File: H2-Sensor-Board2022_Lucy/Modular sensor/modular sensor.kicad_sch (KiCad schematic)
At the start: 6 parts, among them J1 Conn_01x03_Pin

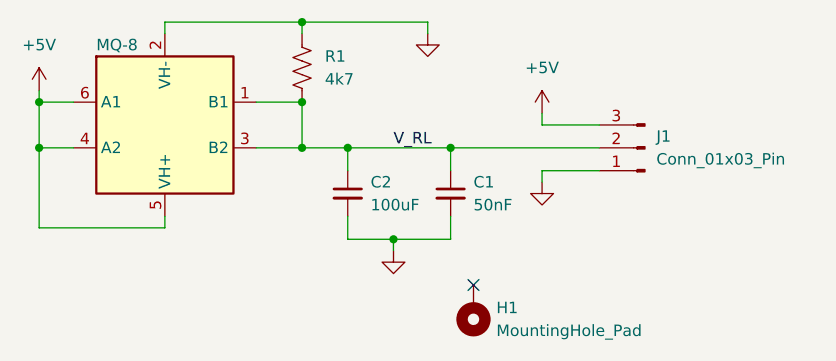
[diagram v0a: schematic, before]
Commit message: I am highly sleep deprived
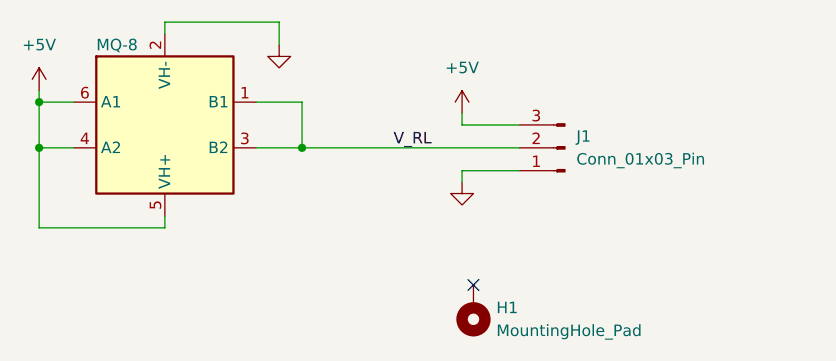
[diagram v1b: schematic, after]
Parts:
- removed C1: 50nF, Capacitor_SMD:C_1206_3216Metric_Pad1.33x1.80mm_HandSolder, symbol Device:C_Small
- removed C2: 100uF, Capacitor_SMD:C_1206_3216Metric_Pad1.33x1.80mm_HandSolder, symbol Device:C_Small
- removed R1: 4k7, Resistor_SMD:R_1206_3216Metric_Pad1.30x1.75mm_HandSolder, symbol Device:R_US
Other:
- moved on the sheet: J1
